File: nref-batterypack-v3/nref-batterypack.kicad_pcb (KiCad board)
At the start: 4 copper layers, 75 x 17 mm, 92 parts, among them J0 C1-, J1 C1-, J2 C2+, J3 C3-, J4 C4+, J5 PACK_CONN, J6 BACK_CONN, Q1 BC817, Q2 BC817, Q3 BC817, Q4 BC817, Q5 AO3401A, Q7 AO3401A, Q8 Q_Dual_NMOS_Picostar_CSD87501L, U1 BQ76922

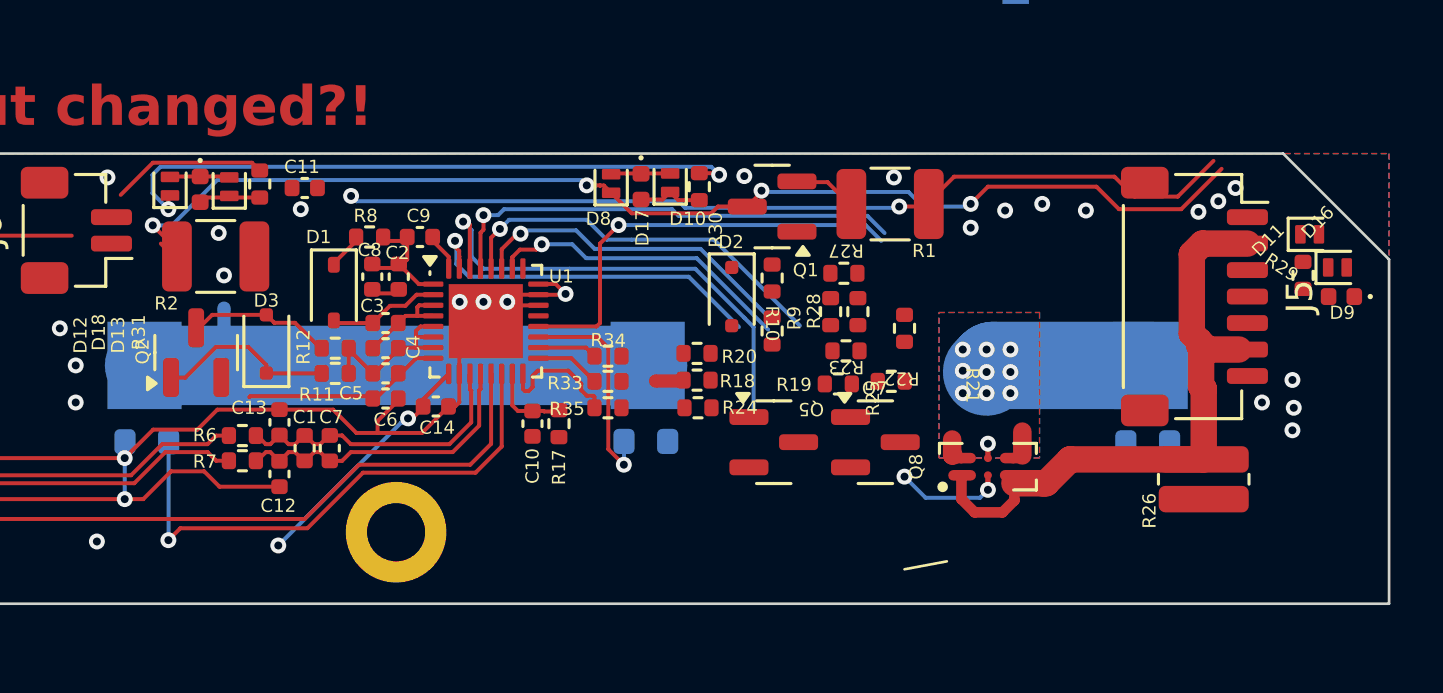
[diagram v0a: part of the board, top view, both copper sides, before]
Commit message: battpack v3 snapshot
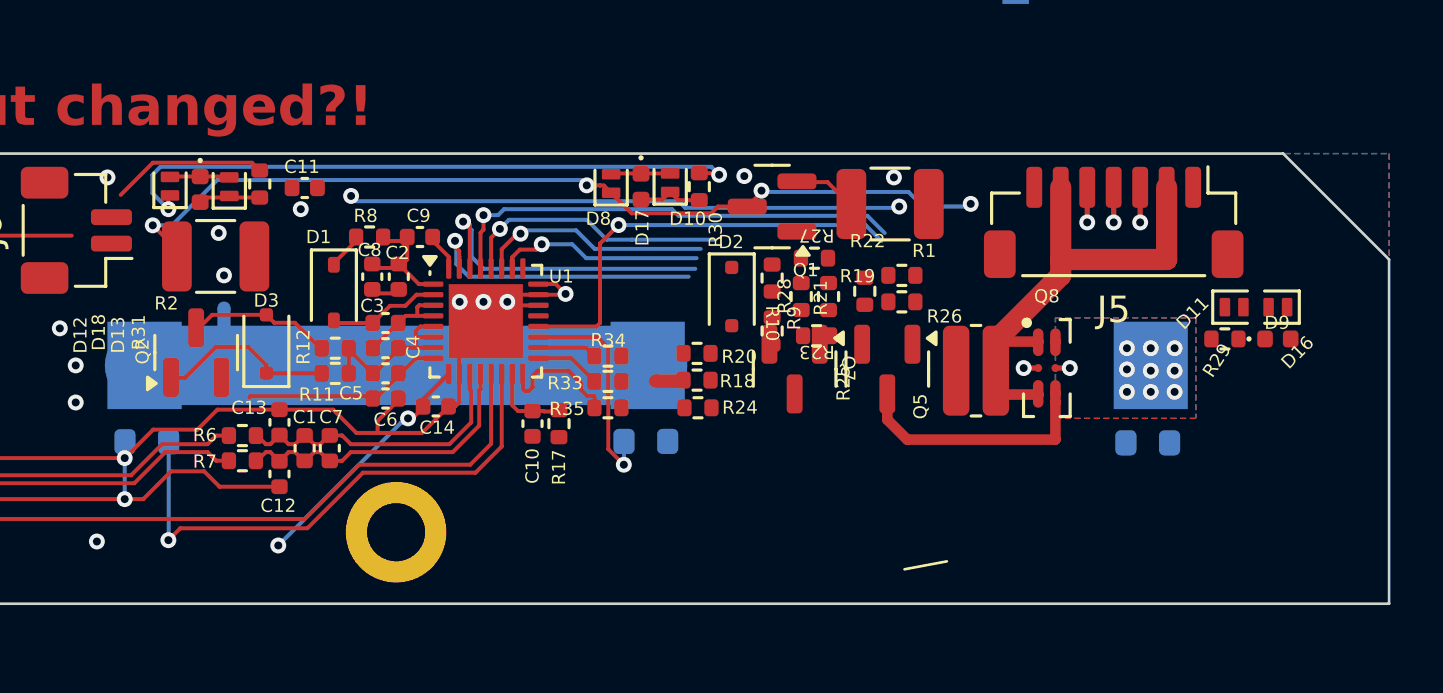
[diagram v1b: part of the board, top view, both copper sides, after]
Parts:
- J5: footprint Connector_JST:JST_SH_SM07B-SRSS-TB_1x07-1MP_P1.00mm_Horizontal -> Connector_JST:JST_SH_BM07B-SRSS-TB_1x07-1MP_P1.00mm_Vertical
- moved R26 9.53 mm to (159.4, 99.2), turned to 0 degrees
- moved Q5 5.10 mm to (156.1, 99.1), turned to -90 degrees
- moved R19 4.75 mm to (156.6, 95.6)
- moved Q8 4.34 mm to (162.1, 99.1), turned to 0 degrees
- moved J5 4.14 mm to (164.6, 93.6), turned to 180 degrees
- moved Q7 4.12 mm to (152.6, 99.1), turned to -90 degrees
- moved D11 3.96 mm to (169.2, 96.8)
- moved R29 3.80 mm to (168.8, 98.0), turned to 180 degrees
- moved R21 3.03 mm to (156.6, 96.6), turned to 180 degrees
- moved D9 2.88 mm to (170.8, 98.0), turned to 0 degrees
- moved D16 2.70 mm to (170.8, 96.8), turned to 180 degrees
- moved R22 2.05 mm to (155.2, 96.2), turned to -90 degrees
- moved R23 1.25 mm to (153.4, 97.9)
- moved R25 1.25 mm to (153.8, 96.4)
- moved R27 1.25 mm to (153.3, 95.0)
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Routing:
- net /VC5: track 38.3 -> 25.1 mm
- net /C3+: track 46.3 -> 34.7 mm
- net /DSG: track 18.5 -> 12.1 mm
- net /LD: track 14.8 -> 10.2 mm
- net /PCHG: track 12.8 -> 8.83 mm
- net /PDSG: track 11.6 -> 7.81 mm
- net /PACK+: track 25.0 -> 21.3 mm
- net Net-(Q8-G1): track 4.16 -> 0.55 mm, vias 2 -> 1
- net /CHG: track 13.7 -> 11.0 mm
- net /SDA: track 0.00 -> 1.32 mm, vias 0 -> 1
- net /SCL: track 0.00 -> 1.32 mm, vias 0 -> 1
- net /ALERT: track 0.00 -> 1.32 mm, vias 0 -> 1
- net /BATplus: track 9.15 -> 10.3 mm
- net GND: vias 39 -> 28
